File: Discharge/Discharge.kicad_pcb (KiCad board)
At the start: 2 copper layers, 77.5 x 49.5 mm, 18 parts, among them J1 TS, J2 Busbar, J3 LV connector, J4 CAN, Q1 2N7002-TP, U1 NE555DR, U2 J1021CS312VDC.20, U3 CPC1008NTR, U4 ZXTR2005ZQ-13

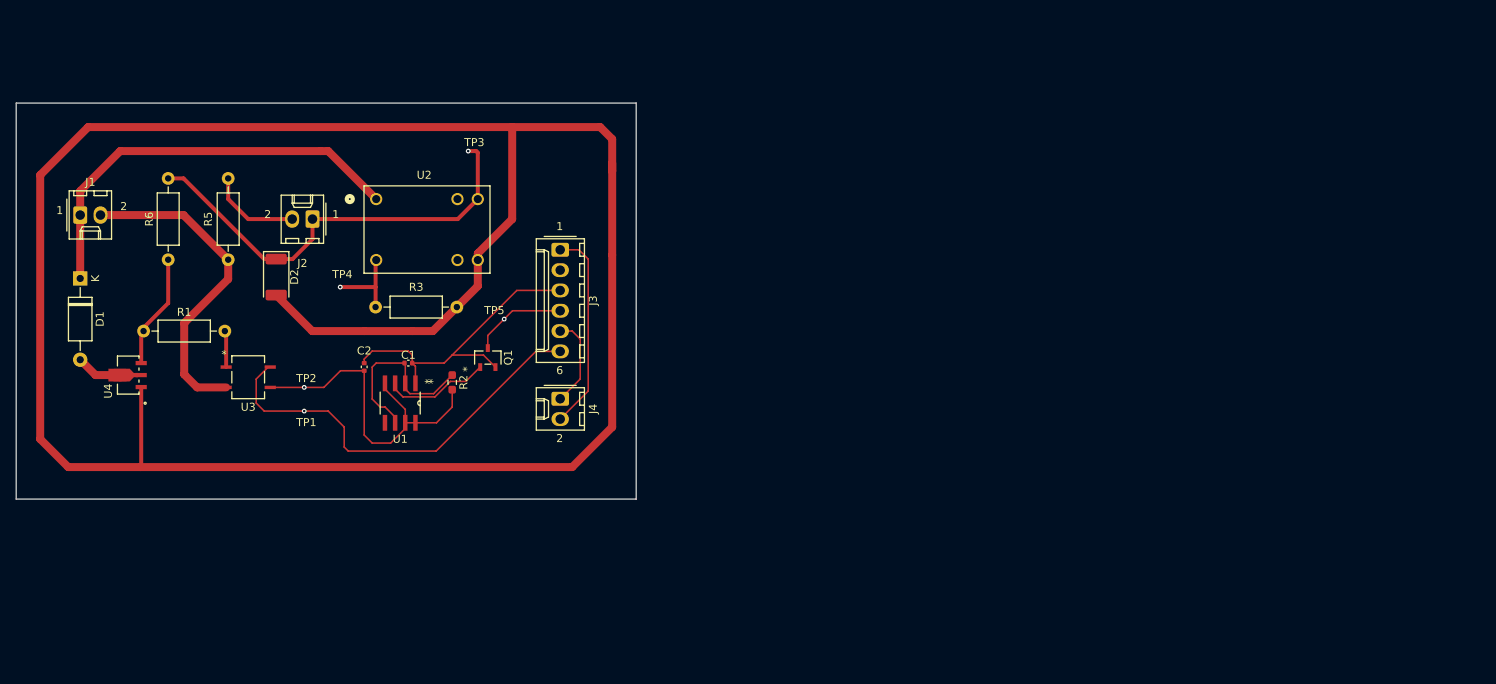
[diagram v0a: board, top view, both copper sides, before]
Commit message: Add files via upload
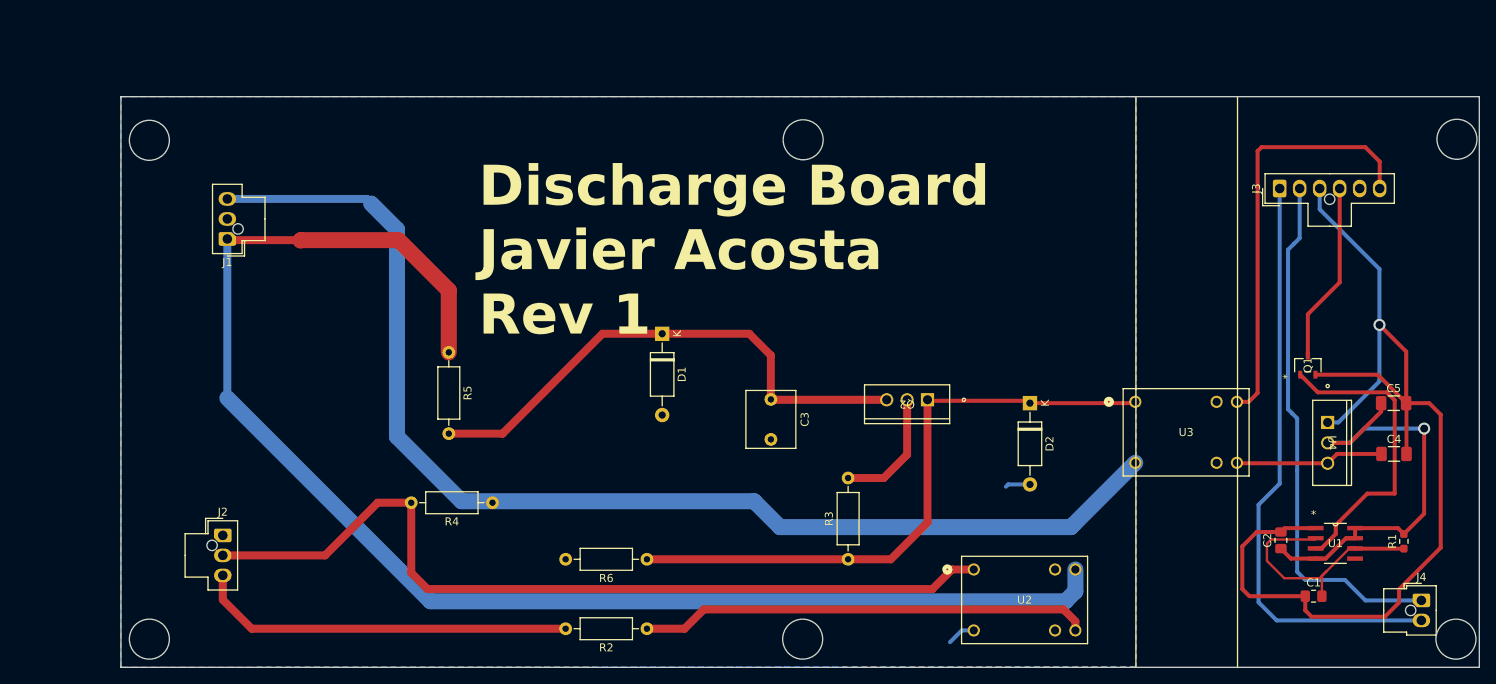
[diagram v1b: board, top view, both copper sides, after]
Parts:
- added C3: 0.1uF, Capacitor_THT:C_Rect_L7.0mm_W6.0mm_P5.00mm, F.Cu at (174.3, 105.5)
- added C4: 100nf, Capacitor_SMD:C_1206_3216Metric_Pad1.33x1.80mm_HandSolder, F.Cu at (252.2, 112.4)
- added C5: 10uf, Capacitor_SMD:C_1206_3216Metric_Pad1.33x1.80mm_HandSolder, F.Cu at (252.2, 106.0)
- added Q2: LD1117V50C, LD1117V50C:TO-220S_STM, F.Cu at (193.9, 105.6)
- added R4: 5k, Resistor_THT:R_Axial_DIN0207_L6.3mm_D2.5mm_P10.16mm_Horizontal, F.Cu at (139.5, 118.5)
- C1, C2: footprint Capacitor_SMD:C_0402_1005Metric -> Capacitor_SMD:C_0805_2012Metric_Pad1.18x1.45mm_HandSolder
- D1: value 60V -> 50v
- D2: value D -> 24v; footprint Diode_SMD:D_2010_5025Metric -> Diode_THT:D_A-405_P10.16mm_Horizontal
- J1, J2: footprint Connector_Molex:Molex_KK-254_AE-6410-02A_1x02_P2.54mm_Vertical -> Connector_Molex:Molex_Nano-Fit_105309-xx03_1x03_P2.50mm_Vertical
- J3: footprint Connector_Molex:Molex_KK-254_AE-6410-06A_1x06_P2.54mm_Vertical -> Connector_Molex:Molex_Nano-Fit_105309-xx06_1x06_P2.50mm_Vertical
- J4: footprint Connector_Molex:Molex_KK-254_AE-6410-02A_1x02_P2.54mm_Vertical -> Connector_Molex:Molex_Nano-Fit_105309-xx02_1x02_P2.50mm_Vertical
- R1: value 15k -> 200k; footprint Resistor_THT:R_Axial_DIN0207_L6.3mm_D2.5mm_P10.16mm_Horizontal -> Resistor_SMD:R_0603_1608Metric_Pad0.98x0.95mm_HandSolder
- R2: value 200k -> 5k; footprint Resistor_SMD:R_0603_1608Metric_Pad0.98x0.95mm_HandSolder -> Resistor_THT:R_Axial_DIN0207_L6.3mm_D2.5mm_P10.16mm_Horizontal
- R3: value 1k -> 220
- R5: value 5k -> 4.7k
- R6: value 5k -> 4k
- U3: value CPC1008NTR -> J1021CS324VDC.20; footprint CPC1008NTR:CPC1008N_IXY -> RelayJ1021:RELAY6_J1021CS312VDC.20_CRS
- U4: value ZXTR2005ZQ-13 -> LD1117V50C; footprint Regulator ZXTR2005ZQ_13:SOT-89_4P5X2P45_DIO -> LD1117V50C:TO-220S_STM
- moved R1 159.7 mm to (253.5, 123.3), turned to 90 degrees
- moved U4 150.0 mm to (243.9, 108.4), turned to -90 degrees
- moved U1 118.2 mm to (244.9, 123.5), turned to 0 degrees
- moved C1 116.8 mm to (242.2, 130.1), turned to 0 degrees
- moved C2 116.6 mm to (238.1, 123.2), turned to 90 degrees
- moved U3 110.9 mm to (219.9, 105.8)
- moved J4 110.6 mm to (255.6, 130.7), turned to 0 degrees
- moved Q1 102.5 mm to (241.5, 101.3)
- moved D2 95.5 mm to (206.7, 106.0)
- moved J3 90.3 mm to (237.9, 79.2), turned to 90 degrees
- moved U2 87.9 mm to (199.7, 126.8)
- moved D1 73.1 mm to (160.7, 97.3)
- moved R6 70.6 mm to (158.8, 125.5), turned to 180 degrees
- moved R3 67.0 mm to (184.0, 125.5), turned to 90 degrees
- moved J2 41.1 mm to (105.8, 122.5), turned to 0 degrees
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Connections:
- C1 pad 1: /GLV -> GLV
- C2 pad 1: /GLV -> Net-(U1-DISCH)
- C2 pad 2: Net-(U1-DISCH) -> GLV
- D1 pad 1: /TS+ -> Net-(D1-K)
- D1 pad 2: Net-(D1-A) -> GND
- D2 pad 1: /MSD (HVD) -> Net-(D2-K)
- J1 pad 2: /TS- -> unconnected-(J1-Pin_2-Pad2)
- J2 pad 1: /MSD (HVD) -> GND
- J2 pad 2: /Shunt Module -> /IR Final
- J3 pad 2: unconnected-(J3-Pin_2-Pad2) -> /CANL
- J3 pad 3: /GLV -> GLV
- J3 pad 5: /CANL -> unconnected-(J3-Pin_5-Pad5)
- Q1 pad 2: /GLV -> GLV
- R1 pad 1: Net-(R1-Pad1) -> Net-(U1-THRES)
- R1 pad 2: Net-(U3-A) -> Net-(U1-DISCH)
- R2 pad 1: Net-(U1-THRES) -> Net-(R2-Pad1)
- R2 pad 2: Net-(U1-DISCH) -> /Shunt Module
- R3 pad 1: Net-(R3-Pad1) -> Net-(D2-K)
- R3 pad 2: GND -> Net-(Q2-VOUT)
- R5 pad 1: /TS- -> /TS+
- R5 pad 2: /Shunt Module -> Net-(D1-K)
- R6 pad 1: Net-(R1-Pad1) -> Net-(D2-K)
- R6 pad 2: /MSD (HVD) -> GND
- U1 pad 1: /GLV -> GLV
- U1 pad 2: unconnected-(U1-TRIG-Pad2) -> Net-(U1-THRES)
- U2 pad 1: /TS+ -> /IR Final
- U2 pad 12: GND -> Net-(R2-Pad1)
- U2 pad 6: /MSD (HVD) -> /TS+
- U2 pad 7: Net-(R3-Pad1) -> GND
- U3 pad 1: Net-(U3-A) -> Net-(D2-K)
- U4 pad 1: GND -> GLV
- U4 pad 2: Net-(D1-A) -> Net-(U1-DISCH)
- U4 pad 3: Net-(R1-Pad1) -> Net-(U4-VIN)
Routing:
- net GND: track 280.7 -> 6.72 mm
- net GLV: track 0.00 -> 135.0 mm, vias 0 -> 1
- net /TS+: track 52.5 -> 177.9 mm
- net /TS-: track 40.8 -> 149.0 mm
- net /IR Final: track 0.00 -> 107.2 mm
- net Net-(D2-K): track 0.00 -> 78.0 mm
- net Net-(D1-K): track 0.00 -> 66.6 mm
- net Net-(R2-Pad1): track 0.00 -> 56.3 mm
- net /CANL: track 11.4 -> 66.0 mm
- net /MSD (HVD): track 54.5 -> 0.00 mm, vias 1 -> 0
- net /CANH: track 25.4 -> 74.1 mm
- net /GLV: track 39.1 -> 0.00 mm
- net /Shunt Module: track 11.7 -> 47.4 mm
- net Net-(Q1-G): track 13.3 -> 38.2 mm
- net Net-(U4-VIN): track 0.00 -> 19.0 mm
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- added copper zone on B.Cu, net GND
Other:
- board size 77.5 x 49.5 mm -> 169.8 x 71.3 mm
- board text added: "Discharge Board Javier Acosta Rev 1"
- board text removed: "1"
- board text removed: "2"
- board text removed: "6"
- board text removed: "TP1"
- board text removed: "TP2"
- board text removed: "TP3"
- board text removed: "TP4"
- board text removed: "TP5"

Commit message: Add files via upload
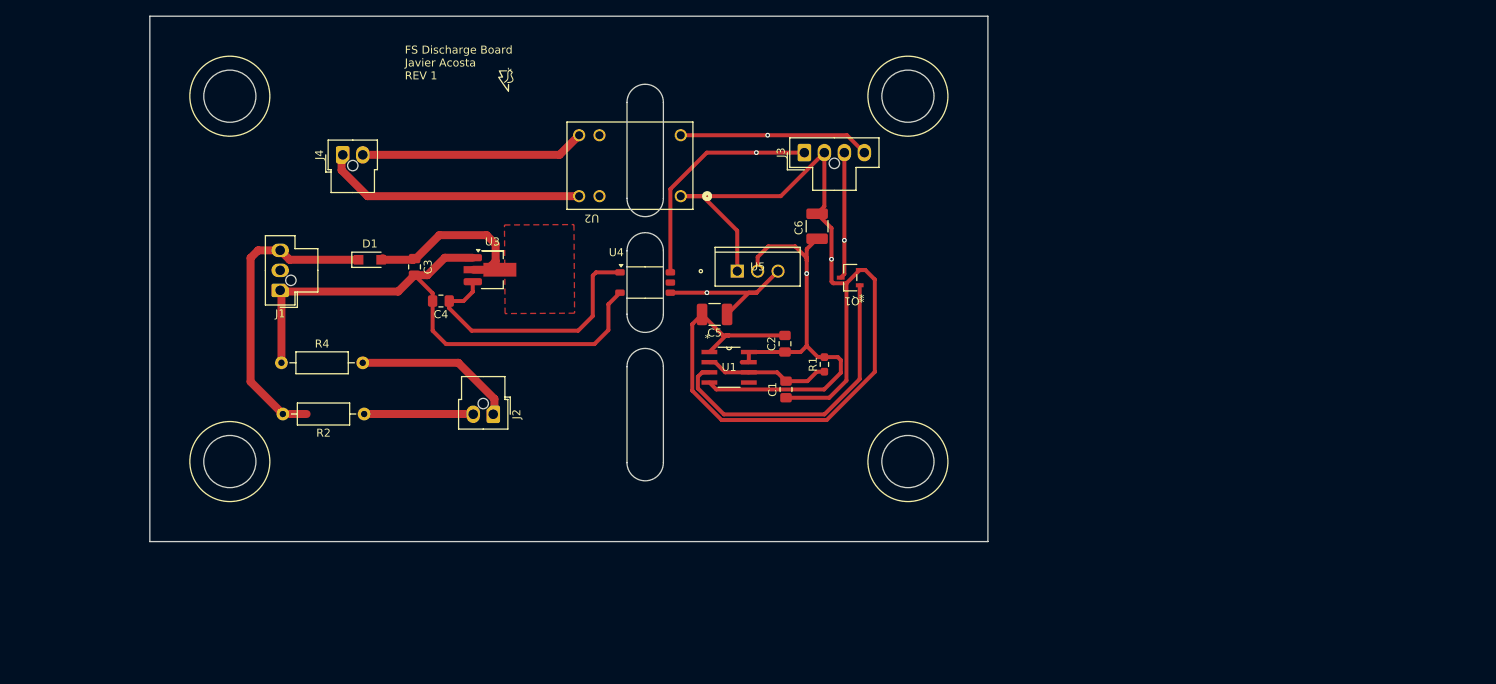
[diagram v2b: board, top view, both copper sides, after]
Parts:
- removed D2: 24v, Diode_THT:D_A-405_P10.16mm_Horizontal
- removed Q2: LD1117V50C, LD1117V50C:TO-220S_STM
- removed R3: 220, Resistor_THT:R_Axial_DIN0207_L6.3mm_D2.5mm_P10.16mm_Horizontal
- removed R5: 4.7k, Resistor_THT:R_Axial_DIN0207_L6.3mm_D2.5mm_P10.16mm_Horizontal
- removed R6: 4k, Resistor_THT:R_Axial_DIN0207_L6.3mm_D2.5mm_P10.16mm_Horizontal
- added C6: 10uF, Capacitor_SMD:C_1210_3225Metric_Pad1.33x2.70mm_HandSolder, F.Cu at (180.1, 83.9)
- added G***: LOGO, FS_3_Global_Footprint_Library:FORMULA SLUG, F.Cu at (144.3, 65.7)
- added U5: LD1117V50C, LD1117V50C:TO-220S_STM, F.Cu at (170.1, 89.5)
- C3: value 0.1uF -> 1uF; footprint Capacitor_THT:C_Rect_L7.0mm_W6.0mm_P5.00mm -> Capacitor_SMD:C_0805_2012Metric_Pad1.18x1.45mm_HandSolder
- C4: value 100nf -> 10uF; footprint Capacitor_SMD:C_1206_3216Metric_Pad1.33x1.80mm_HandSolder -> Capacitor_SMD:C_0805_2012Metric_Pad1.18x1.45mm_HandSolder
- C5: value 10uf -> 100nF; footprint Capacitor_SMD:C_1206_3216Metric_Pad1.33x1.80mm_HandSolder -> Capacitor_SMD:C_1210_3225Metric_Pad1.33x2.70mm_HandSolder
- D1: value 50v -> 50V; footprint Diode_THT:D_A-405_P10.16mm_Horizontal -> Diode_SMD:Nexperia_CFP3_SOD-123W
- J2: value Busbar -> TSMP; footprint Connector_Molex:Molex_Nano-Fit_105309-xx03_1x03_P2.50mm_Vertical -> Connector_Molex:Molex_Nano-Fit_105309-xx02_1x02_P2.50mm_Vertical
- J3: value LV connector -> Conn_01x06; footprint Connector_Molex:Molex_Nano-Fit_105309-xx06_1x06_P2.50mm_Vertical -> Connector_Molex:Molex_Nano-Fit_105309-xx04_1x04_P2.50mm_Vertical
- J4: value CAN -> Conn_01x02
- U3: value J1021CS324VDC.20 -> ZXTR2005ZQ-13; footprint RelayJ1021:RELAY6_J1021CS312VDC.20_CRS -> Package_TO_SOT_SMD:SOT-89-3_Handsoldering
- U4: value LD1117V50C -> TLP3122AE; footprint LD1117V50C:TO-220S_STM -> Package_SO:SO-5-6_4.55x3.7mm_P1.27mm
- moved J4 145.9 mm to (120.8, 75.0), turned to 90 degrees
- moved C4 120.7 mm to (133.1, 93.2), turned to 180 degrees
- moved U4 87.1 mm to (158.6, 90.9), turned to 0 degrees
- moved C5 85.6 mm to (167.3, 94.9), turned to 180 degrees
- moved U3 82.0 mm to (139.5, 89.3)
- moved U1 78.9 mm to (169.1, 101.5)
- moved R1 75.7 mm to (181.0, 101.2)
- moved C1 70.8 mm to (176.2, 104.3), turned to 90 degrees
- moved C2 66.7 mm to (176.1, 98.6)
- moved J3 59.6 mm to (178.5, 74.7)
- moved U2 59.3 mm to (163.1, 80.1), turned to 180 degrees
- moved Q1 58.2 mm to (184.3, 90.3), turned to 180 degrees
- moved C3 47.5 mm to (129.8, 89.0)
- moved R2 44.4 mm to (123.5, 107.4)
- moved D1 37.7 mm to (124.2, 88.1), turned to 0 degrees
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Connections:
- C3 pad 1: Net-(D1-K) -> Net-(D1-A)
- C3 pad 2: GND -> /TS-
- C4 pad 1: Net-(U4-VIN) -> Net-(U3-VO)
- C4 pad 2: GLV -> /TS-
- C5 pad 1: Net-(U1-DISCH) -> Net-(U5-VIN)
- D1 pad 1: Net-(D1-K) -> /TS+
- D1 pad 2: GND -> Net-(D1-A)
- J1 pad 1: /TS+ -> /TS-
- J1 pad 3: /TS- -> /TS+
- J2 pad 1: GND -> /TSMP-
- J2 pad 2: /IR Final -> /TSMP+
- J3 pad 1: /CANH -> 12v
- J3 pad 2: /CANL -> GLV
- J3 pad 3: GLV -> /RTM
- J3 pad 4: /RTM -> /IR Final
- J4 pad 1: /CANL -> /Discharge-
- J4 pad 2: /CANH -> /Discharge+
- R2 pad 1: Net-(R2-Pad1) -> /TSMP+
- R2 pad 2: /Shunt Module -> /TS+
- R4 pad 2: /IR Final -> /TSMP-
- U2 pad 1: /IR Final -> GLV
- U2 pad 12: Net-(R2-Pad1) -> /Discharge+
- U2 pad 6: /TS+ -> /Discharge-
- U2 pad 7: GND -> /IR Final
- U3 pad 1: Net-(D2-K) -> /TS-
- U4 pad 1: GLV -> Net-(U3-VO)
- U4 pad 3: Net-(U4-VIN) -> /TS-
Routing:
- net /TS+: track 177.9 -> 38.5 mm
- net /IR Final: track 107.2 -> 23.9 mm, vias 0 -> 1
- net Net-(D2-K): track 78.0 -> 0.00 mm
- net /TS-: track 149.0 -> 71.8 mm
- net /CANH: track 74.1 -> 0.00 mm
- net Net-(D1-K): track 66.6 -> 0.00 mm
- net /CANL: track 66.0 -> 0.00 mm
- net Net-(R2-Pad1): track 56.3 -> 0.00 mm
- net /Shunt Module: track 47.4 -> 0.00 mm
- net Net-(U3-VO): track 0.00 -> 34.1 mm
- net /Discharge-: track 0.00 -> 33.0 mm
- net /Discharge+: track 0.00 -> 28.1 mm
- net 12v: track 52.9 -> 29.3 mm, vias 0 -> 1
- net Net-(D1-A): track 0.00 -> 21.7 mm
- net /TSMP-: track 0.00 -> 20.3 mm
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- added copper zone on F.Cu, net Net-(D1-A)
- removed copper zone on B.Cu, net GND
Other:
- board size 169.8 x 71.3 mm -> 104.8 x 65.7 mm
- board text added: "FS Discharge Board Javier Acosta REV 1"
- board text removed: "Discharge Board Javier Acosta Rev 1"

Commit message: Add files via upload
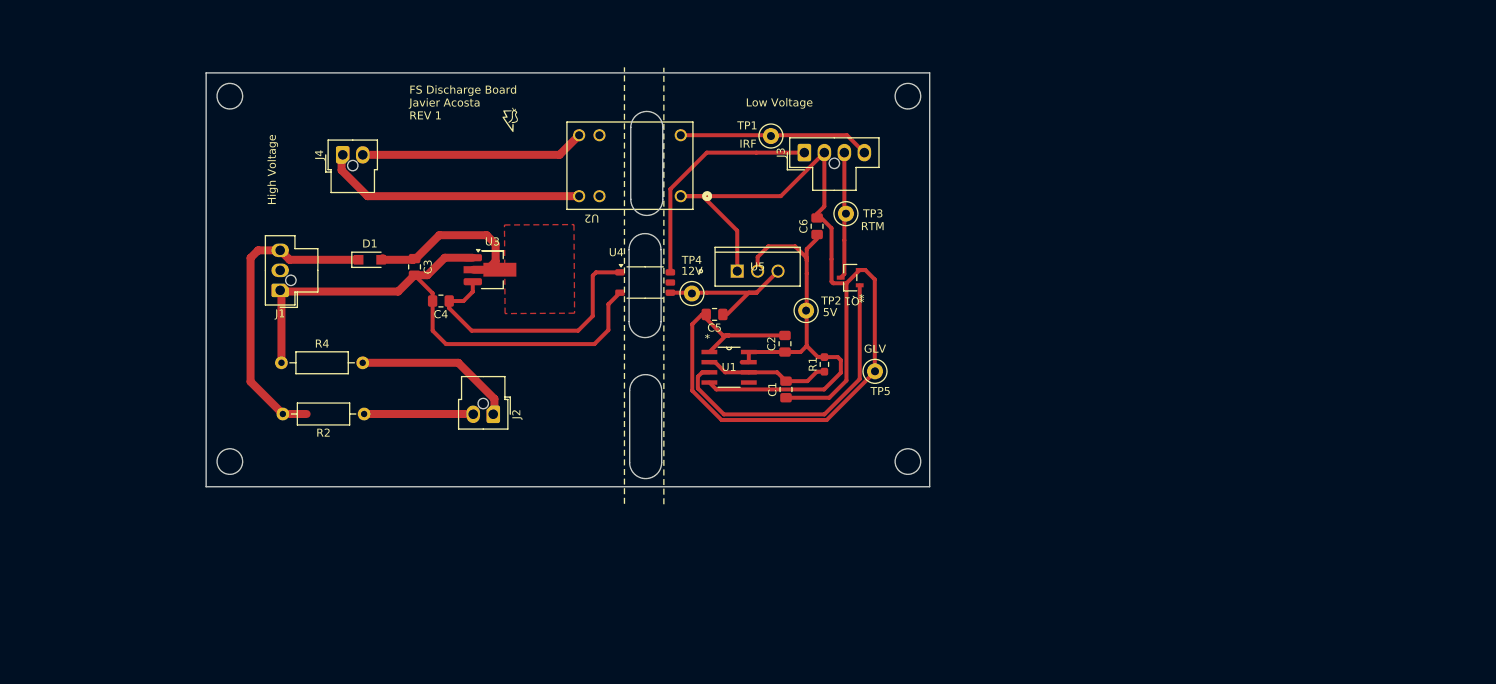
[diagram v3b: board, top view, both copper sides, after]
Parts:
- added TP1: IRF, TestPoint:TestPoint_Loop_D2.50mm_Drill1.0mm, F.Cu at (174.3, 72.6)
- added TP2: 5V, TestPoint:TestPoint_Loop_D2.50mm_Drill1.0mm, F.Cu at (178.7, 94.4)
- added TP3: RTM, TestPoint:TestPoint_Loop_D2.50mm_Drill1.0mm, F.Cu at (183.7, 82.3)
- added TP4: 12V, TestPoint:TestPoint_Loop_D2.50mm_Drill1.0mm, F.Cu at (164.5, 92.3)
- added TP5: GLV, TestPoint:TestPoint_Loop_D2.50mm_Drill1.0mm, F.Cu at (187.4, 102.0)
- C5, C6: footprint Capacitor_SMD:C_1210_3225Metric_Pad1.33x2.70mm_HandSolder -> Capacitor_SMD:C_0805_2012Metric_Pad1.18x1.45mm_HandSolder
- moved G*** 5.03 mm to (144.9, 70.7)
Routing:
- net Net-(U5-VIN): vias 1 -> 0
- net Net-(U1-DISCH): vias 1 -> 0
- net GLV: vias 1 -> 0
- net 12v: vias 1 -> 0
- net /RTM: vias 1 -> 0
- net /IR Final: vias 1 -> 0
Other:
- board size 104.8 x 65.7 mm -> 90.4 x 51.7 mm
- board text added: "High Voltage"
- board text added: "Low Voltage"
